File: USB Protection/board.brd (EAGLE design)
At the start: 25.4 x 17.8 mm, 5 parts, among them J1 USB-MB-H

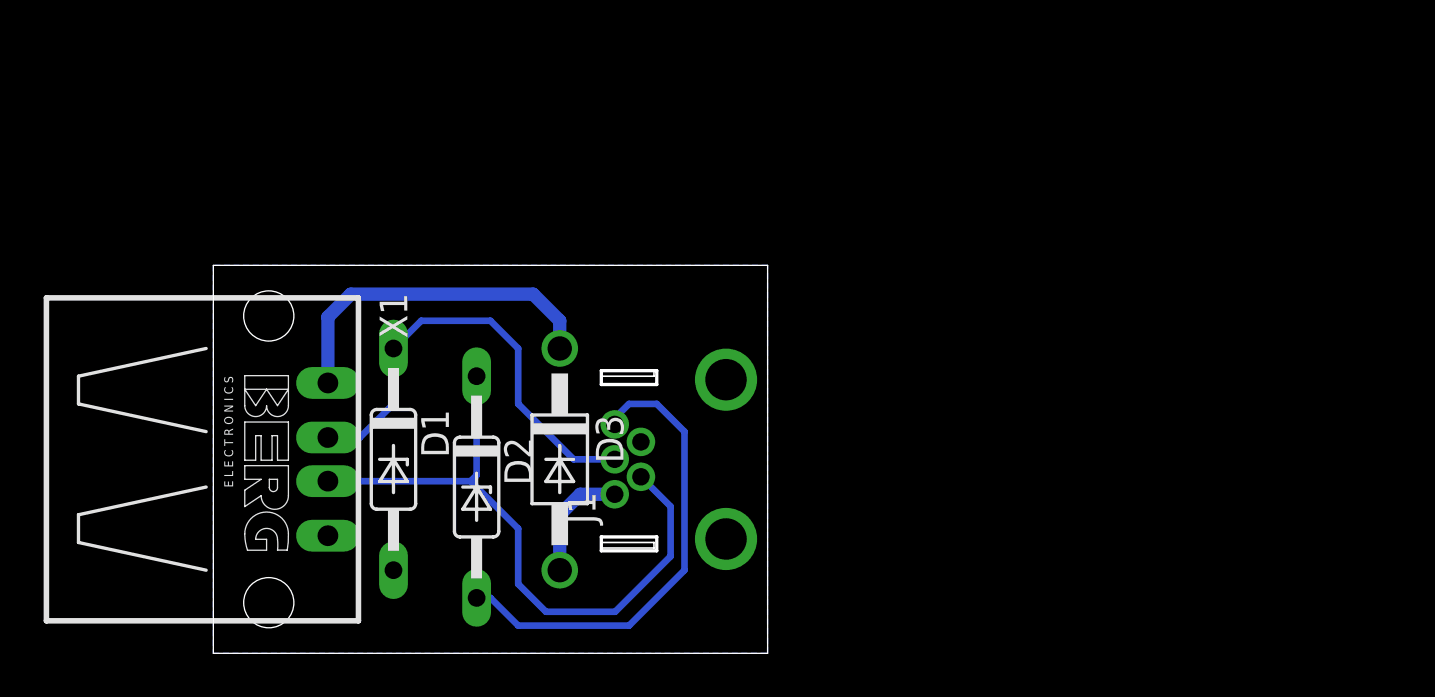
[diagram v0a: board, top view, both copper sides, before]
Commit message: Added lab 6
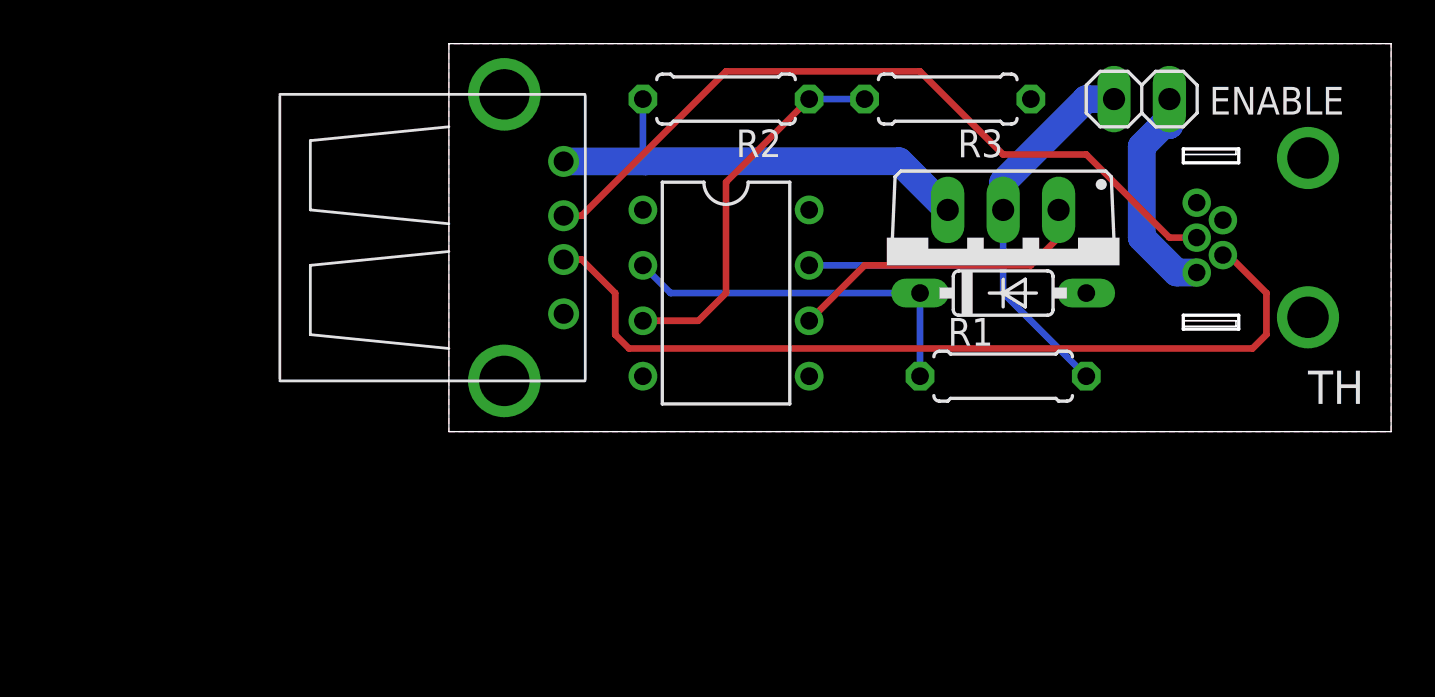
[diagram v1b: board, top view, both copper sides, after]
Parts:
- removed D1, D2: 1N821, diode:DO35Z10
- removed X1: (no value), con-berg:PN87520
- added ENABLE: (no value), pinhead:1X02
- added IC1: LM741P, linear:DIL08
- added Q1: (no value), transistor-power:TO220BV
- added R1: 560, resistor:0207/7
- added R2, R3: (no value), resistor:0207/7
- added USB_A: (no value), con-usb-3:USB-A-H
- D3: value 1N4942 -> BZX55Z2V0; device diode:DO41-10 -> diode:DO35-7
- moved J1 28.5 mm to (55.9, 22.9)
- moved D3 21.7 mm to (41.9, 20.3), turned to 0 degrees
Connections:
- removed net N$1: D3.C, X1.1
- new net VBUS_IN: ENABLE.1, J1.VBUS
- new net VREF: D3.C, IC1.2, R1.1
- new net V_EDIV: IC1.3, R2.1, R3.2
- new net V_EN: IC1.6, Q1.G
- new net V_EXT: Q1.S, R2.2, USB_A.VBUS
- net D+: now also USB_A.D+; no longer D2.C, X1.3
- net D-: now also USB_A.D-; no longer D1.C, X1.2
- net GND: now also D3.A, IC1.4, R3.1, USB_A.GND; no longer D1.A, D2.A, X1.4
- net VBUS: now also ENABLE.2, IC1.7, Q1.D, R1.2; no longer D3.A, J1.VBUS
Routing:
- net GND: track 21.7 -> 0.00 mm
- net V_EXT: track 0.00 -> 21.4 mm
- net VBUS: track 5.45 -> 26.0 mm
- net V_EDIV: track 0.00 -> 17.3 mm
- net VREF: track 0.00 -> 17.0 mm
- net N$1: track 15.9 -> 0.00 mm
- net V_EN: track 0.00 -> 14.3 mm
- net D-: track 21.0 -> 34.9 mm
- net VBUS_IN: track 0.00 -> 10.2 mm
- net D+: track 29.9 -> 39.9 mm
- added copper zone on layer 1, net GND
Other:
- board size 25.4 x 17.8 mm -> 43.2 x 17.8 mm
- board text added: "TH"
